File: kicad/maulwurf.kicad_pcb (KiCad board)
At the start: 2 copper layers, 63.5 x 70 mm, 17 parts

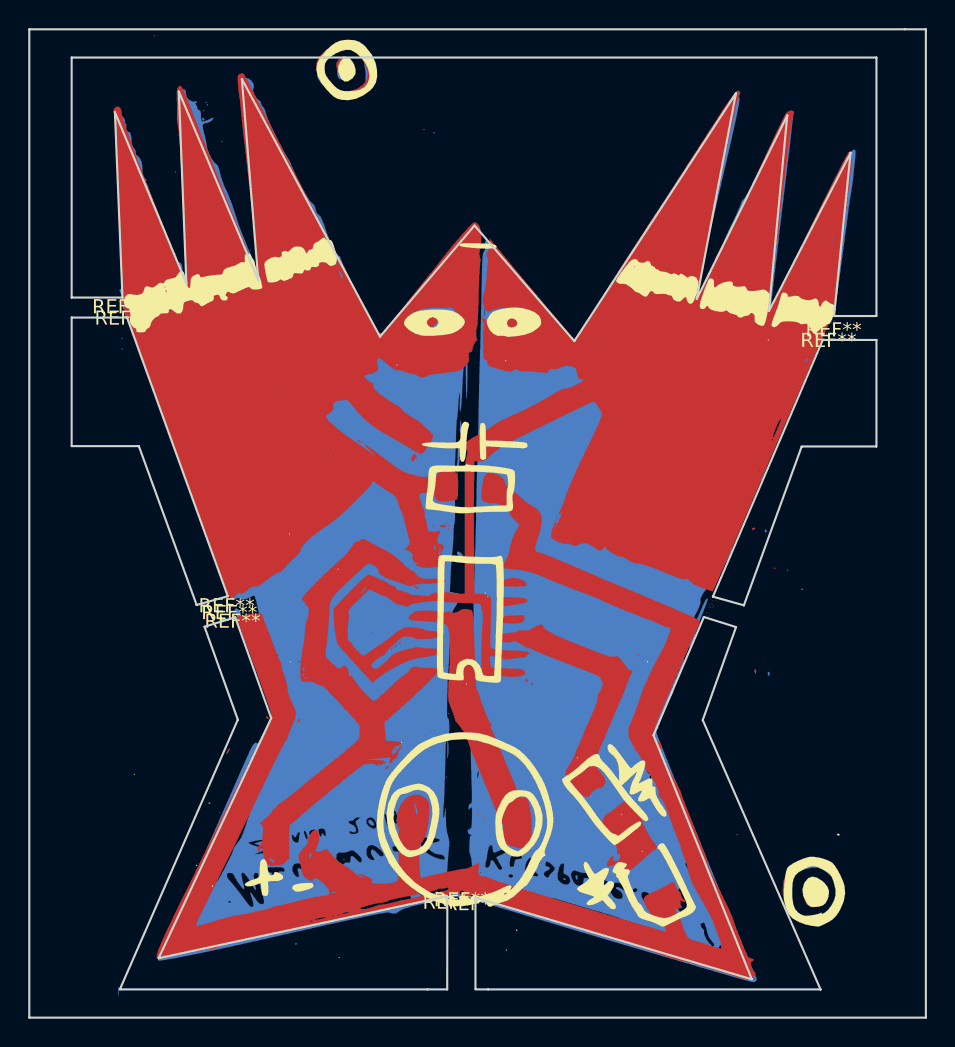
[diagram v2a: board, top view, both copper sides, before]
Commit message: Improve rat-bites
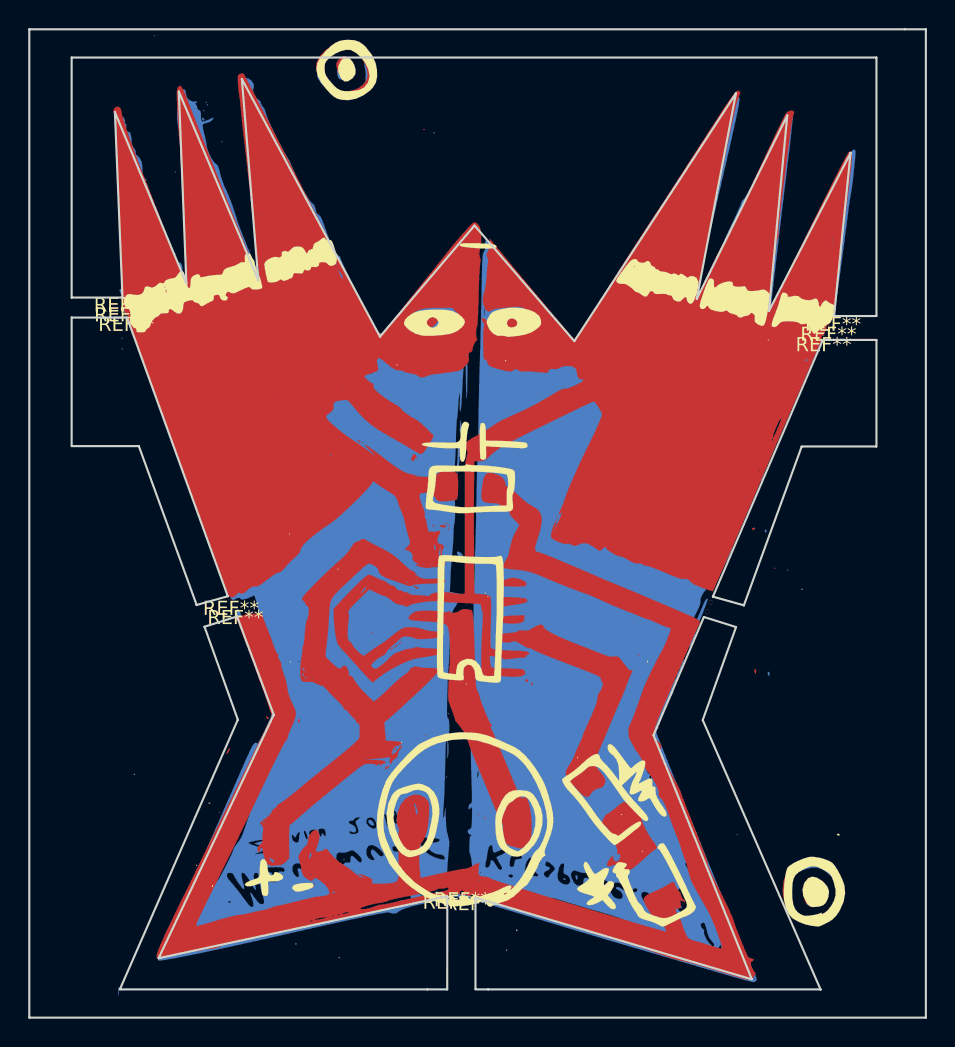
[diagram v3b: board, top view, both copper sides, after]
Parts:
- removed the REF** at (156.5, 100.4)
- removed the REF** at (122.4, 101.4)
- added REF**: hole, footprints:hole, F.Cu at (114.6, 79.7)
- added REF**: hole, footprints:hole, F.Cu at (164.6, 81.1)
- moved REF** 0.55 mm to (122.6, 101.2)
- moved REF** 0.51 mm to (114.9, 80.4)
- moved REF** 0.46 mm to (164.3, 81.8)
- moved REF** 0.40 mm to (164.9, 80.4)
- moved REF** 0.36 mm to (122.3, 100.5)
- moved REF** 0.26 mm to (156.3, 100.6)
- moved REF** 0.22 mm to (156.0, 101.2)
- moved REF** 0.18 mm to (114.6, 79.0)
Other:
- outline, holes or cut-outs redrawn
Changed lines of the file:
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@@
     (links 0)
     (no_connects 0)
-    (area 107.924999 59.924999 171.575001 130.075001)
+    (area 107.924999 55.664333 171.575001 130.075001)
     (thickness 1.6)
     (drawings 57)
@@
     (uvia_drill 0.1)
   )
-  (module footprints:hole (layer B.Cu)
-    (at 156.489477 100.350167 180)
-    (fp_text reference REF** (at 0 -0.5 180) (layer B.SilkS)
-      (effects (font (size 1 1) (thickness 0.15)) (justify mirror))
+  (module footprints:hole (layer F.Cu)
+    (at 114.578 79.725)
+    (fp_text reference REF** (at 0 0.5) (layer F.SilkS)
+      (effects (font (size 1 1) (thickness 0.15)))
     )
-    (fp_text value hole (at 0 0.5 180) (layer B.Fab)
-      (effects (font (size 1 1) (thickness 0.15)) (justify mirror))
+    (fp_text value hole (at 0 -0.5) (layer F.Fab)
+      (effects (font (size 1 1) (thickness 0.15)))
     )
-    (pad 1 thru_hole circle (at 0 0 180) (size 0.3 0.3) (drill 0.3) (layers *.Cu *.Mask))
+    (pad 1 thru_hole circle (at 0 0) (size 0.3 0.3) (drill 0.3) (layers *.Cu *.Mask))
+  )
+  (module footprints:hole (layer F.Cu)
+    (at 164.599 81.101)
+    (fp_text reference REF** (at 0 0.5) (layer F.SilkS)
+      (effects (font (size 1 1) (thickness 0.15)))
+    )
+    (fp_text value hole (at 0 -0.5) (layer F.Fab)
+      (effects (font (size 1 1) (thickness 0.15)))
+    )
+    (pad 1 thru_hole circle (at 0 0) (size 0.3 0.3) (drill 0.3) (layers *.Cu *.Mask))
   )
   (module footprints:hole (layer B.Cu)
-    (at 156.071477 101.446167 180)
+    (at 156.01 101.236 180)
     (fp_text reference REF** (at 0 -0.5 180) (layer B.SilkS)
       (effects (font (size 1 1) (thickness 0.15)) (justify mirror))
@@
   )
   (module footprints:hole (layer B.Cu)
-    (at 156.298477 100.837167 180)
+    (at 156.284 100.578 180)
     (fp_text reference REF** (at 0 -0.5 180) (layer B.SilkS)
       (effects (font (size 1 1) (thickness 0.15)) (justify mirror))
@@
   )
   (module footprints:hole (layer F.Cu)
-    (at 121.976 100.325)
-    (fp_text reference REF** (at 0 0.5) (layer F.SilkS)
-      (effects (font (size 1 1) (thickness 0.15)))
-    )
-    (fp_text value hole (at 0 -0.5) (layer F.Fab)
-      (effects (font (size 1 1) (thickness 0.15)))
-    )
-    (pad 1 thru_hole circle (at 0 0) (size 0.3 0.3) (drill 0.3) (layers *.Cu *.Mask))
-  )
-  (module footprints:hole (layer F.Cu)
-    (at 122.394 101.421)
+    (at 122.284 100.511)
     (fp_text reference REF** (at 0 0.5) (layer F.SilkS)
       (effects (font (size 1 1) (thickness 0.15)))
@@
   )
   (module footprints:hole (layer F.Cu)
-    (at 122.167 100.812)
+    (at 122.596 101.163)
     (fp_text reference REF** (at 0 0.5) (layer F.SilkS)
       (effects (font (size 1 1) (thickness 0.15)))
@@
   )
   (module footprints:hole (layer F.Cu)
-    (at 114.608 79.958)
+    (at 114.866 80.401)
     (fp_text reference REF** (at 0 0.5) (layer F.SilkS)
       (effects (font (size 1 1) (thickness 0.15)))
@@
   )
   (module footprints:hole (layer F.Cu)
-    (at 114.434 79.151)
+    (at 114.558 79.024)
     (fp_text reference REF** (at 0 0.5) (layer F.SilkS)
       (effects (font (size 1 1) (thickness 0.15)))
@@
   )
   (module footprints:hole (layer F.Cu)
-    (at 164.965 80.785)
+    (at 164.929 80.391)
     (fp_text reference REF** (at 0 0.5) (layer F.SilkS)
       (effects (font (size 1 1) (thickness 0.15)))
@@
   )
   (module footprints:hole (layer F.Cu)
-    (at 164.605 81.535)
+    (at 164.253 81.837)
     (fp_text reference REF** (at 0 0.5) (layer F.SilkS)
       (effects (font (size 1 1) (thickness 0.15)))
@@
   (gr_line (start 155.777 101.622) (end 158.055477 102.338167) (layer Edge.Cuts) (width 0.15))
   (gr_line (start 155.698477 108.926167) (end 164.047477 128.017167) (layer Edge.Cuts) (width 0.15))
-  (gr_line (start 125.131 108.783) (end 122.586 101.65) (layer Edge.Cuts) (width 0.15))
+  (gr_line (start 125.322 108.571) (end 122.713 101.576) (layer Edge.Cuts) (width 0.15))
   (gr_line (start 122.774 108.909) (end 120.409 102.314) (layer Edge.Cuts) (width 0.15))
-  (gr_line (start 122.584 101.648) (end 120.41 102.313) (layer Edge.Cuts) (width 0.15))
+  (gr_line (start 122.724 101.582) (end 120.41 102.313) (layer Edge.Cuts) (width 0.15))
   (gr_line (start 119.84 100.775) (end 122.058 100.155) (layer Edge.Cuts) (width 0.15))
   (gr_line (start 122.767 108.901) (end 114.418 127.992) (layer Edge.Cuts) (width 0.15))
@@
   (gr_line (start 140.5 128) (end 164.04501 128) (layer Edge.Cuts) (width 0.15))
   (gr_line (start 111 80.409988) (end 111 89.525) (layer Edge.Cuts) (width 0.15))
-  (gr_line (start 117.158 125.793) (end 125.138 108.784) (layer Edge.Cuts) (width 0.15))
+  (gr_line (start 117.158 125.793) (end 125.312 108.551) (layer Edge.Cuts) (width 0.15))
   (gr_line (start 137.6 121.4) (end 117.158 125.793) (layer Edge.Cuts) (width 0.15))
   (gr_line (start 159.174 127.286) (end 139.6 121.5) (layer Edge.Cuts) (width 0.15))
